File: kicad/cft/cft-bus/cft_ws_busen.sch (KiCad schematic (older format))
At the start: 42 parts, among them U22 ICS501, U34 74LVC1G32, U42 74HC08, U43 74LVC1G04, U44 74LVC1G3208, U45 74LVC1G125, U46 74AHC1G32, U47 74LVC1G74, U48 74ACT245, U49 74LVC1G11, U50 74ACT245, U52 74LVC1G17, U53 74LVC1G373

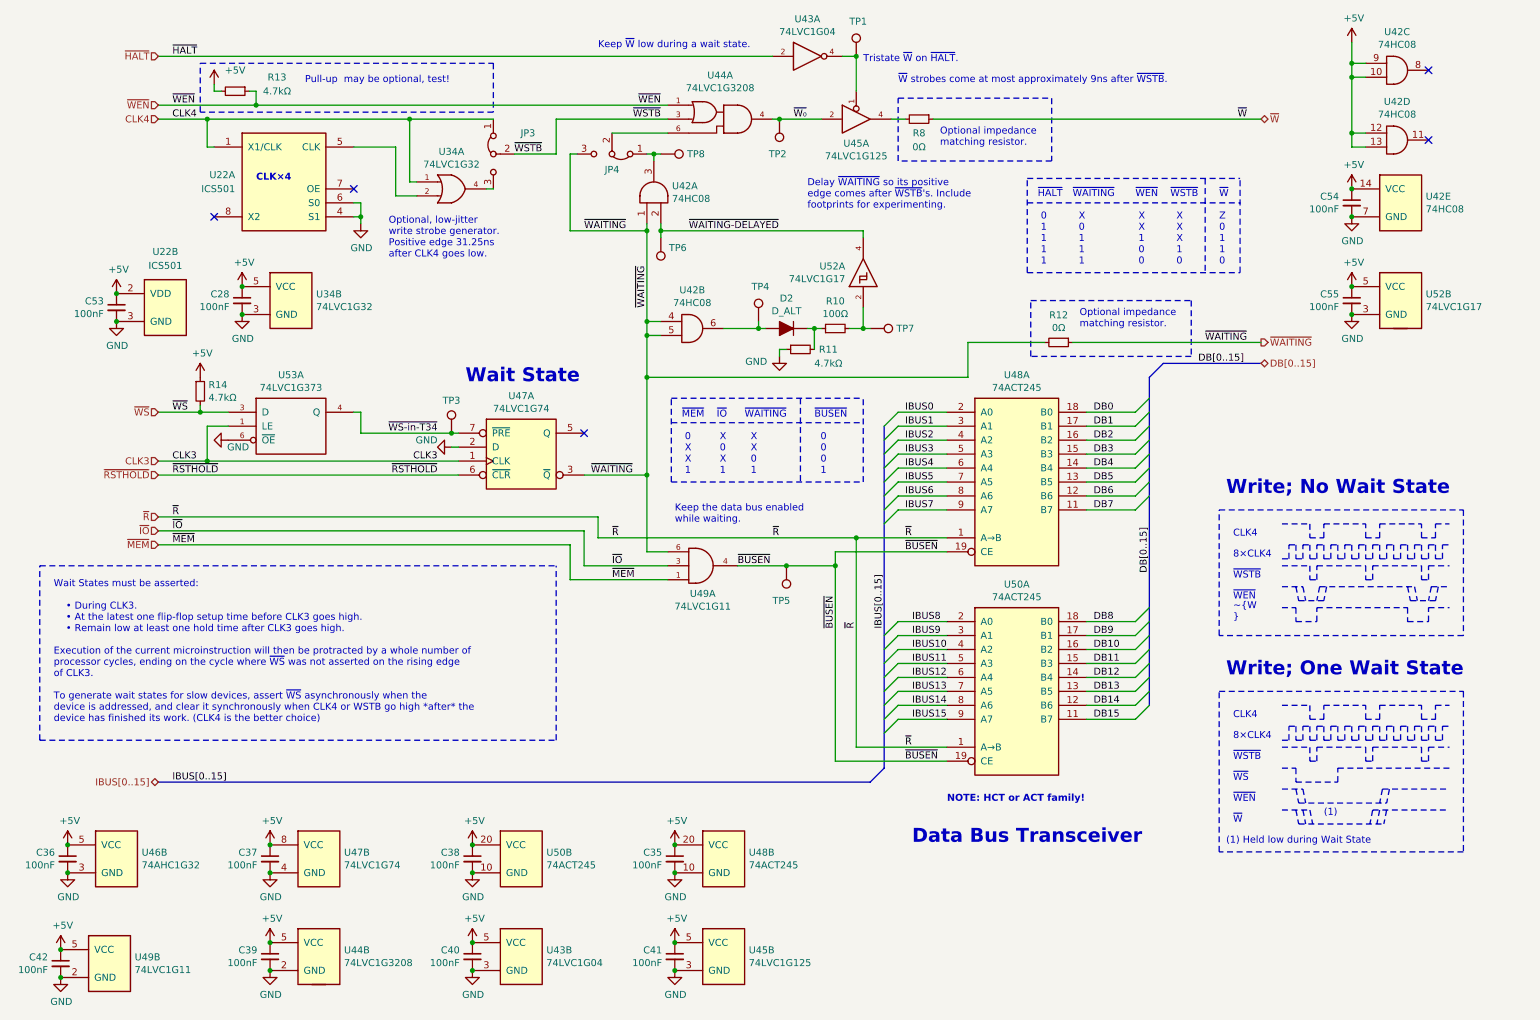
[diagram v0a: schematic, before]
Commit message: Worked out simpler Wait State and Write drivers.
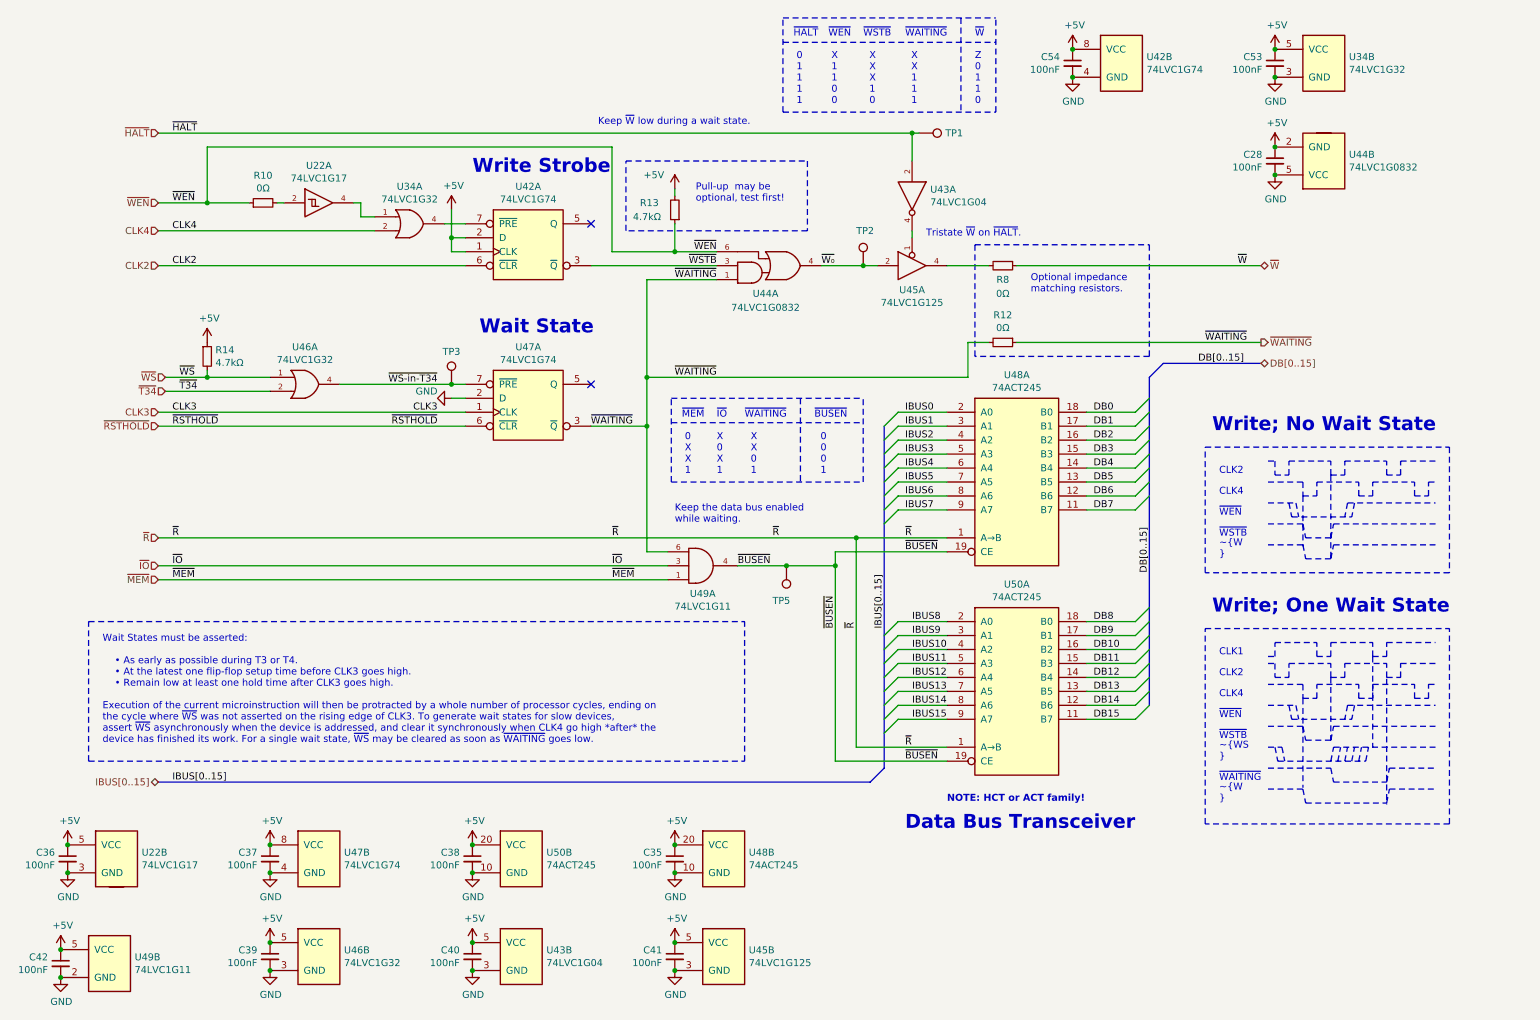
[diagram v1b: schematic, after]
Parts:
- removed C55: 100nF, alexios:C_SMD_0805_2012Metric_Pad1.15x1.40mm_HandSolder, symbol Device:C_Small
- removed D2: D_ALT, alexios:SOD-323, symbol Device:D_ALT
- removed JP3, JP4: Jumper_3_Bridged12, Jumper:SolderJumper-3_P1.3mm_Bridged12_RoundedPad1.0x1.5mm, symbol Jumper:Jumper_3_Bridged12
- removed R11: 4.7kΩ, alexios:R_SMD_0805_2012Metric_Pad1.15x1.40mm_HandSolder, symbol Device:R_Small
- removed TP4, TP6, TP7, TP8: TestPoint, TestPoint:TestPoint_Pad_1.0x1.0mm, symbol Connector:TestPoint
- removed U22: ICS501, alexios:SOIC-8, symbol alexios:ICS501
- removed U42: 74HC08, alexios:SOIC-14, symbol alexios:74HC08
- removed U44: 74LVC1G3208, alexios:SOT-23-6_Handsoldering, symbol alexios:74LVC1G3208
- removed U46: 74AHC1G32, alexios:SOT-23-5_HandSoldering, symbol alexios:74AHC1G32
- removed U52: 74LVC1G17, alexios:SOT-23-5_HandSoldering, symbol alexios:74LVC1G17
- removed U53: 74LVC1G373, alexios:SOT-23-6_Handsoldering, symbol alexios:74LVC1G373
- added U22: 74LVC1G17, alexios:SOT-23-5_HandSoldering, symbol alexios:74LVC1G17
- added U42: 74LVC1G74, alexios:TSSOP-8_3x3mm_P0.65mm, symbol alexios:74AUC1G74
- added U44: 74LVC1G0832, alexios:SOT-23-6_Handsoldering, symbol alexios:74LVC1G0832
- added U46: 74LVC1G32, alexios:SOT-23-5_HandSoldering, symbol alexios:74LVC1G32
- R10: value 100Ω -> 0Ω
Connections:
- net +5V: now also U22.5 (VCC), U42.1 (CLK), U42.2 (D), U42.8 (VCC), U44.2 (GND), U46.5 (VCC)
- net CLK4: now also U34.2; no longer U34.1
- net GND: now also U22.3 (GND), U42.4 (GND), U44.5 (VCC), U46.3 (GND)
- net ~HALT: now also TP1.1
- net ~WAITING: now also U44.1
- net ~WEN: now also R10.1, U44.6
- net ~WS: now also U46.1
- net ~WS-in-T34: now also U46.4
- net ~WSTB: now also U42.3 (~Q), U44.3
- net ~W₀: now also U44.4
- net at U43.4, U45.1: no longer TP1.1
- net at R10.2: now also U22.2
- net at U34.4: now also U42.7 (~PRE)
- new net: U22.4, U34.1
- new net CLK2: U42.6 (~CLR)
- new net ~T34: U46.2
- no-connect marks 5 -> 2
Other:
- note added: "CLK1"
- note added: "CLK2"
- note added: "Optional impedance\nmatching resistors."
- note added: "Pull-up may be\noptional, test first!"
- note added: "Wait States must be asserted:\n\n • As early as possible during T3 or T4.\n • At the latest one flip-flop setup time before CLK3 goes high.\n • Remain low at least one hold time after CLK3 goes high.\n\nExecution of the current microinstruction will then be protracted by a whole number of processor cycles, ending on\nthe cycle where ~WS~ was not asserted on the rising edge of CLK3. To generate wa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"
- note added: "Write Strobe"
- note added: "~IO~\n\nX\n0\nX\n1"
- note added: "~WAITING"
- note added: "~WAITING~\n\n X\n X\n 1\n 1\n 1"
- note added: "~WEN~\n\n X\n 1\n 1\n 0\n 0"
- note added: "~WS\n"
- note removed: "(1)"
- note removed: "(1) Held low during Wait State"
- note removed: "8×CLK4"
- note removed: "CLK×4"
- note removed: "Delay ~WAITING~ so its positive\nedge comes after ~WSTB~'s. Include\nfootprints for experimenting."
- note removed: "Optional impedance\nmatching resistor."
- note removed: "Optional, low-jitter\nwrite strobe generator.\nPositive edge 31.25ns\nafter CLK4 goes low."
- note removed: "Pull-up may be optional, test!"
- note removed: "Wait States must be asserted:\n\n • During CLK3.\n • At the latest one flip-flop setup time before CLK3 goes high.\n • Remain low at least one hold time after CLK3 goes high.\n\nExecution of the current microinstruction will then be protracted by a whole number of\nprocessor cycles, ending on the cycle where ~WS~ was not asserted on the rising edge\nof CLK3.\n\nTo generate wait states for slow de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"
- note removed: "~IO~\n\n X\n 0\n X\n 1"
- note removed: "~WAITING~\n\n X\n 0\n 1\n 1\n 1"
- note removed: "~WEN~\n\n X\n X\n 1\n 0\n 0"
- note removed: "~WS~"
- note removed: "~W~"
- note removed: "~W~ strobes come at most approximately 9ns after ~WSTB~."
- moved on the sheet: R12, R13, R14, R8, TP1, TP2, TP3, U43A, U45A, U47A
